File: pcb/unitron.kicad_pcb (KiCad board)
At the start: 2 copper layers, 80.3 x 155 mm, 86 parts, among them J1 Conn_01x10_Male, J2 Conn_01x10_Female, J3 Conn_01x10_Male, J4 Conn_01x10_Female, SW1 SPST_B12AP, SW2 SW_SPST, U1 LTC-4727JS, U2 LTC-4727JS, U3 AS1115-BSST, U4 QT_Py, U5 MCP73831-2-OT, U6 LTC-4727JR, U7 LTC-4727JR, U8 AS1115-BSST

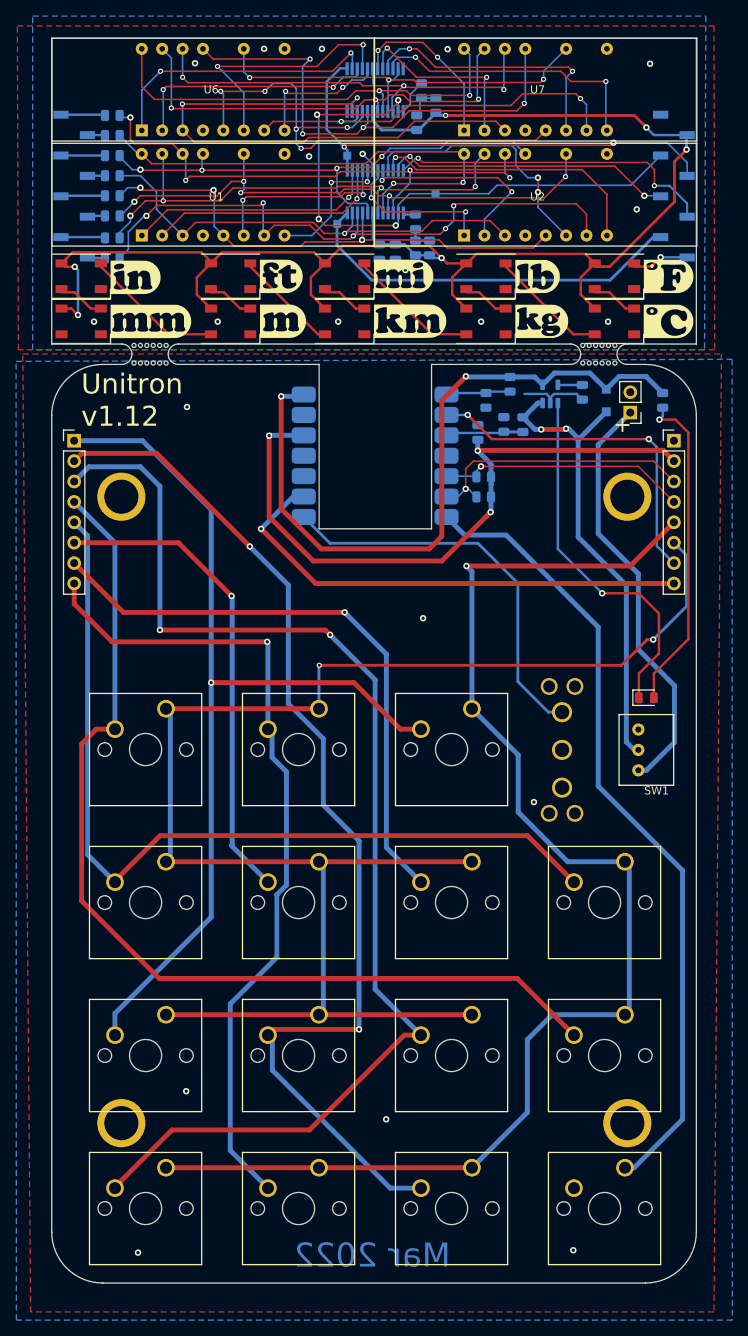
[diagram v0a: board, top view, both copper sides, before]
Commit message: pcb v1.13
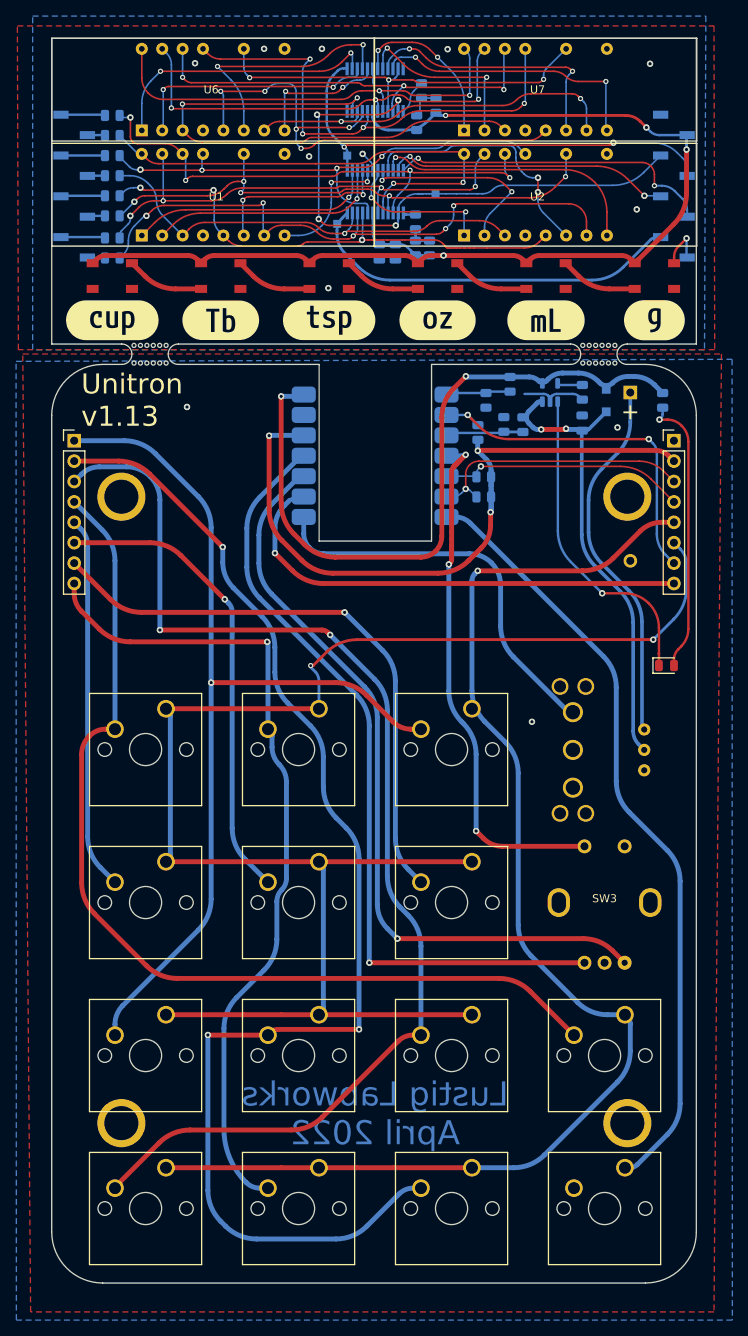
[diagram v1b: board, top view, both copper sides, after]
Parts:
- removed D10, D9: WS2812B, LED_SMD:LED_WS2812B_PLCC4_5.0x5.0mm_P3.2mm
- removed the D7 at (86.2, 52.5)
- removed the D8 at (86.2, 58.1)
- removed G*** (x10): LOGO, LOGO
- removed the S6 at (135.3, 125.4)
- added C3: 10µF, Capacitor_SMD:C_0805_2012Metric, B.Cu at (130.0, 70.8)
- added SW3: RotaryEncoder_Switch, asl_footprints:encoder_PEC11R, F.Cu at (132.8, 130.5)
- added kibuzzard-6260D796: G***, kibuzzard-6260D796, F.Cu at (98.5, 58.0)
- added kibuzzard-6260D7DE: G***, kibuzzard-6260D7DE, F.Cu at (112.0, 58.0)
- added kibuzzard-6260D82F: G***, kibuzzard-6260D82F, F.Cu at (125.5, 58.0)
- added kibuzzard-6260D857: G***, kibuzzard-6260D857, F.Cu at (139.0, 58.0)
- added kibuzzard-6260D976: G***, kibuzzard-6260D976, F.Cu at (85.0, 58.0)
- added kibuzzard-6260DA5E: G***, kibuzzard-6260DA5E, F.Cu at (71.5, 58.0)
- SW1: value SPST_B12AP -> SPST
- U5: value MCP73831-2-OT -> MCP73831
- moved D6 29.5 mm to (71.5, 52.5)
- moved D4 20.3 mm to (98.5, 52.5)
- moved D5 15.4 mm to (85.0, 52.5)
- moved D2 10.2 mm to (125.5, 52.5)
- moved D3 6.03 mm to (112.0, 52.5)
- moved D1 4.97 mm to (139.0, 52.5)
- moved D8 4.72 mm to (140.5, 101.0)
- moved BT1 2.50 mm to (136.0, 67.0), turned to 0 degrees
- moved SW2 1.35 mm to (128.9, 111.5)
- moved SW1 1.27 mm to (136.7, 111.5), turned to 0 degrees
- moved U5 0.18 mm to (126.0, 67.0)
- renumbered D11 to D7, D12 to D8, S11 to S10, S12 to S11, S13 to S12, S14 to S13, S15 to S14, S7 to S6, S8 to S7, S9 to S8, S10 to S9
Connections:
- D6 pad 2: Net-(D6-Pad2) -> unconnected-(D6-Pad2)
- U4 pad 10: unconnected-(U4-Pad10) -> /encoder_b
- U4 pad 11: unconnected-(U4-Pad11) -> /encoder_a
- U4 pad 4: unconnected-(U4-Pad4) -> /encoder_btn
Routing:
- net /encoder_a: track 0.00 -> 98.7 mm, vias 0 -> 1
- net /encoder_b: track 0.00 -> 95.6 mm, vias 0 -> 1
- net /encoder_btn: track 0.00 -> 65.5 mm, vias 0 -> 3
- net Net-(J2-Pad5): track 109.0 -> 46.7 mm
- net /VIN_daughter: track 188.0 -> 142.1 mm, vias 6 -> 4
- net Net-(J2-Pad2): track 133.7 -> 159.4 mm, vias 2 -> 3
- net Net-(D8-Pad2) (its old number): track 17.2 -> 0.00 mm
- net Net-(D6-Pad2): track 12.8 -> 0.00 mm
- net /KEYA: track 167.8 -> 161.1 mm
- net Net-(D4-Pad2): track 16.2 -> 9.66 mm
- net Net-(BT1-Pad1): track 52.6 -> 46.2 mm
- net Net-(D10-Pad4): track 5.74 -> 0.00 mm
- net Net-(D7-Pad2): track 5.74 -> 0.00 mm
- net Net-(D8-Pad1): track 45.6 -> 39.9 mm
- net Net-(D8-Pad2): track 40.7 -> 35.2 mm
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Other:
- outline, holes or cut-outs redrawn
- board text added: "IRQ"
- board text added: "Lustig Labworks April 2022"
- board text added: "R4-R11"
- board text added: "Unitron v1.13"
- board text added: "v1.13"
- board text removed: "Mar 2022"
- board text removed: "Unitron v1.12"
- board text removed: "v1.12"
